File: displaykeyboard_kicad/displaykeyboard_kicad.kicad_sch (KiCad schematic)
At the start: 22 parts, among them SW1 SW_PUSH, SW2 SW_PUSH, SW3 SW_PUSH, SW4 SW_PUSH, SW5 SW_PUSH, SW6 SW_PUSH, SW7 SW_PUSH, SW8 SW_PUSH, SW9 SW_PUSH, U0 supermini_RNF52840, U1 TCA9548APWR, U2 TCA9548APWR, U3 MCP73871

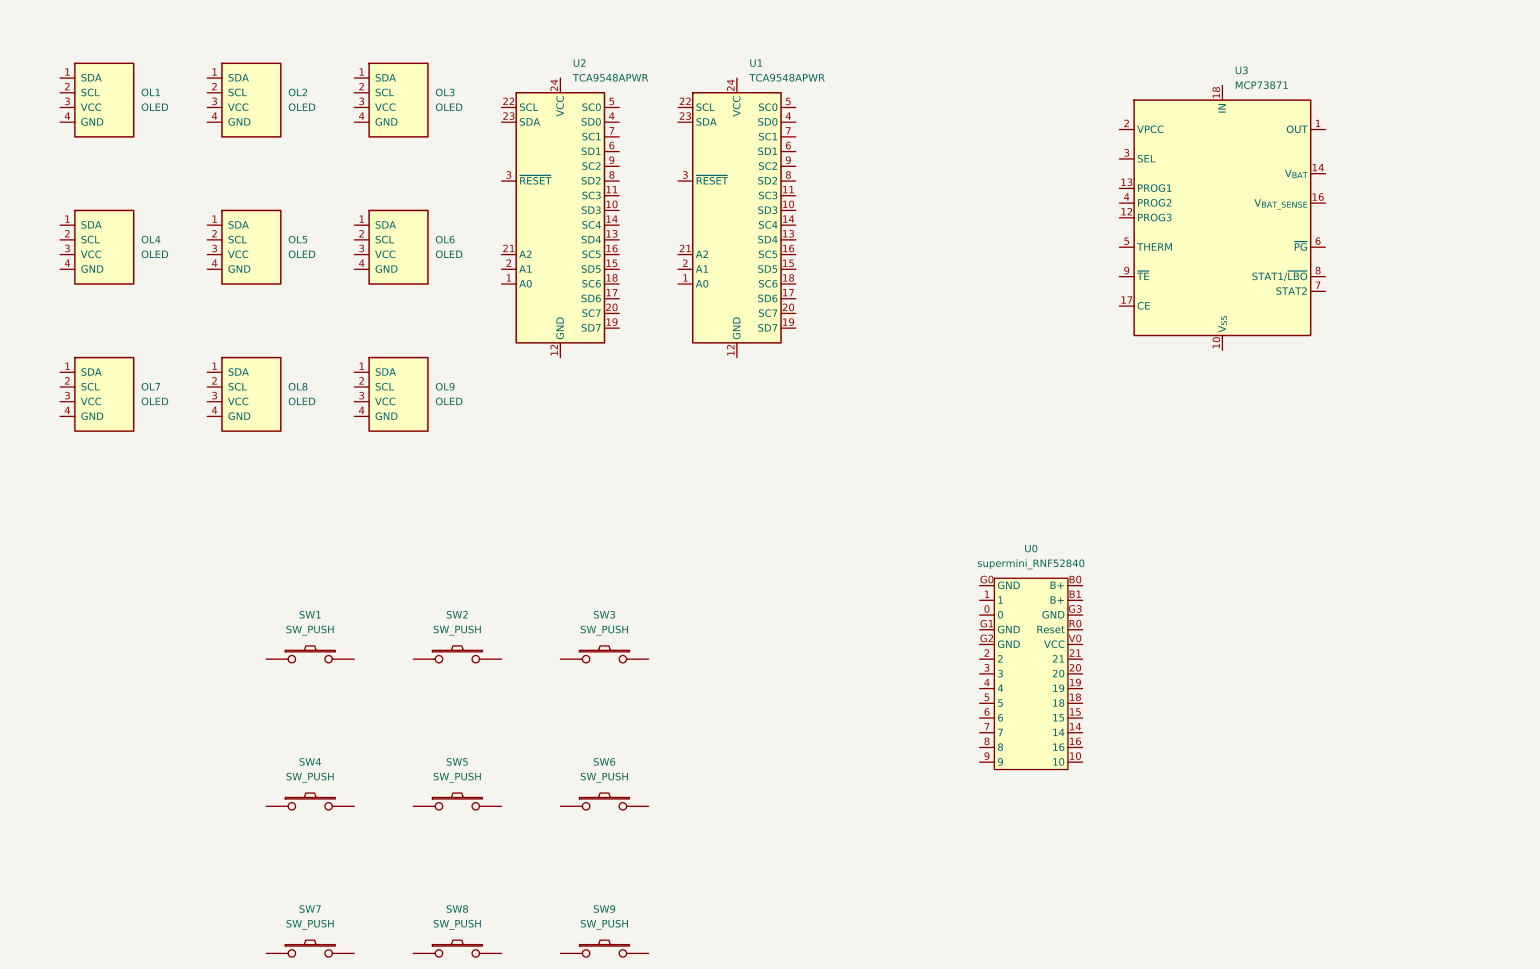
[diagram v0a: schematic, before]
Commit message: main
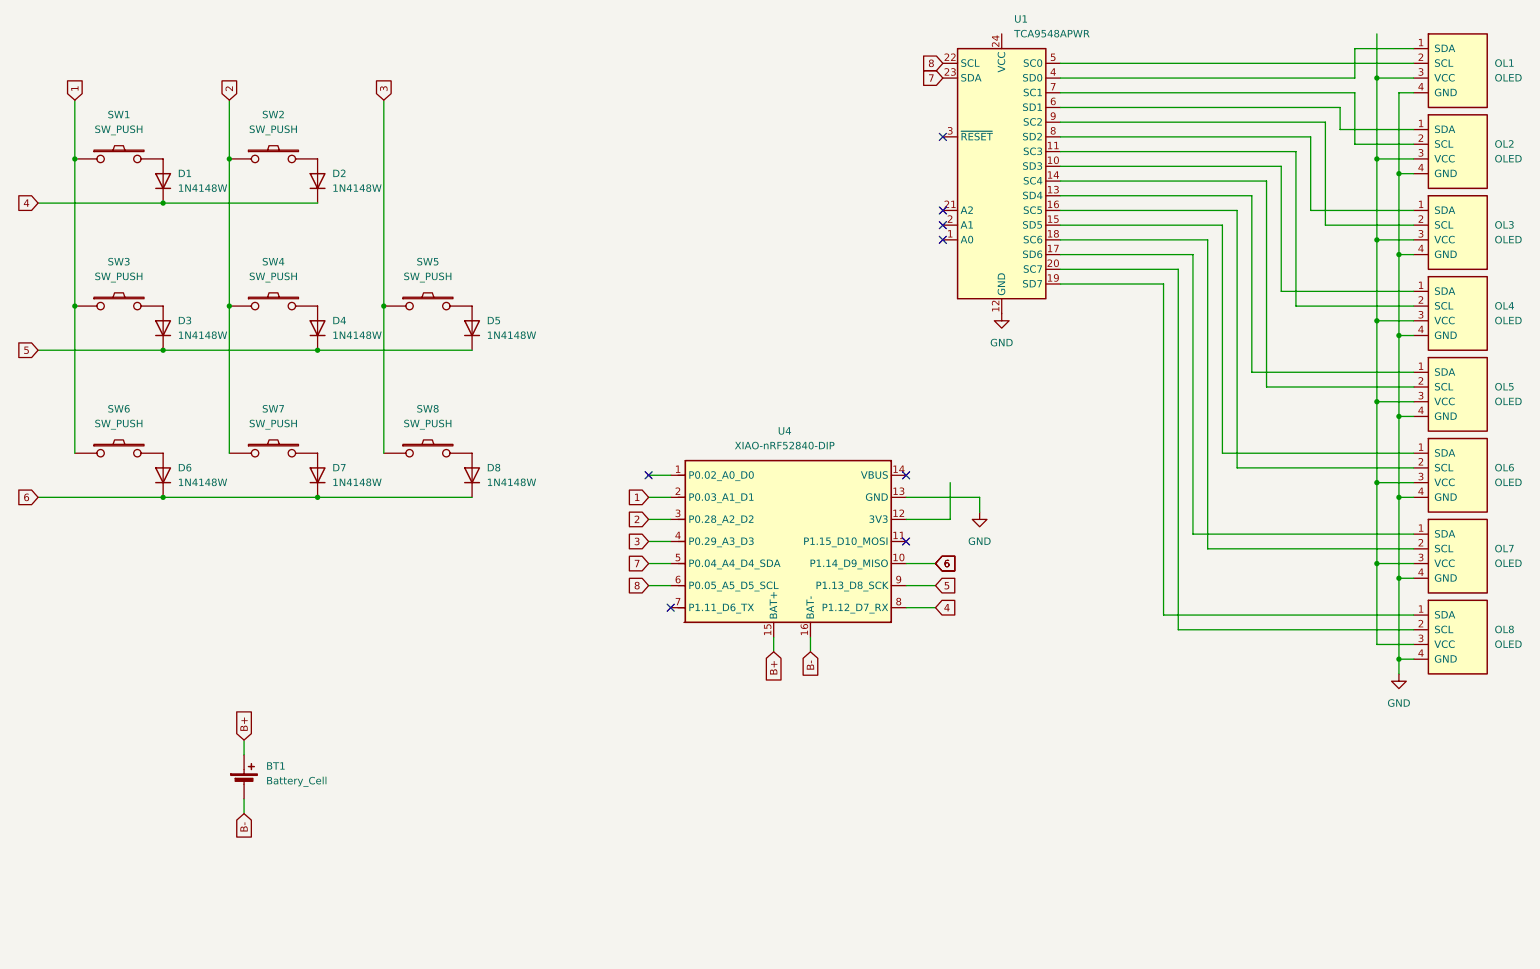
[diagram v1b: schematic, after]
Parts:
- removed OL9: OLED, symbol BrownSugar_KBD:OLED
- removed SW9: SW_PUSH, symbol BrownSugar_KBD:SW_PUSH
- removed U0: supermini_RNF52840, symbol superMini:supermini_NRF52840
- removed U2: TCA9548APWR, Package_SO:TSSOP-24_4.4x7.8mm_P0.65mm, symbol Interface_Expansion:TCA9548APWR
- removed U3: MCP73871, Package_DFN_QFN:QFN-20-1EP_4x4mm_P0.5mm_EP2.5x2.5mm, symbol Battery_Management:MCP73871
- added BT1: Battery_Cell, symbol Device:Battery_Cell
- added D1, D2, D3, D4, D5, D6, D7, D8: 1N4148W, Diode_SMD:D_SOD-123, symbol Diode:1N4148W
- added U4: XIAO-nRF52840-DIP, Seeed_Studio_XIAO_Series:XIAO-nRF52840-DIP, symbol Seeed_Studio_XIAO_Series:XIAO-nRF52840-DIP
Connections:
- net at OL6.1 (SDA): now also U1.15 (SD5)
- net at OL6.2 (SCL): now also U1.16 (SC5)
- net at OL6.3 (VCC): now also OL1.3 (VCC), OL2.3 (VCC), OL3.3 (VCC), OL4.3 (VCC), OL5.3 (VCC), OL7.3 (VCC), OL8.3 (VCC)
- net GND: now reaches OL6.4 (GND)
- net GND: now also OL1.4 (GND), OL2.4 (GND), OL3.4 (GND), OL4.4 (GND), OL5.4 (GND), OL7.4 (GND), OL8.4 (GND), U1.12 (GND), U4.13 (GND)
- net at OL7.1 (SDA): now also U1.17 (SD6)
- net at OL7.2 (SCL): now also U1.18 (SC6)
- net at OL3.1 (SDA): now also U1.8 (SD2)
- net at OL3.2 (SCL): now also U1.9 (SC2)
- net 1: now reaches SW1.1
- net 1: now also SW3.1, SW6.1, U4.2 (P0.03_A1_D1)
- net at SW1.2: now also D1.2 (A)
- net at OL5.1 (SDA): now also U1.13 (SD4)
- net at OL5.2 (SCL): now also U1.14 (SC4)
- net at SW6.2: now also D6.2 (A)
- net at SW3.2: now also D3.2 (A)
- net 3: now reaches SW8.1
- net 3: now also SW5.1, U4.4 (P0.29_A3_D3)
- net at SW8.2: now also D8.2 (A)
- net 2: now reaches SW4.1
- net 2: now also SW2.1, SW7.1, U4.3 (P0.28_A2_D2)
- net at SW4.2: now also D4.2 (A)
- net at OL2.1 (SDA): now also U1.6 (SD1)
- net at OL2.2 (SCL): now also U1.7 (SC1)
- net at SW5.2: now also D5.2 (A)
- net at SW2.2: now also D2.2 (A)
- net at OL1.1 (SDA): now also U1.4 (SD0)
- net at OL1.2 (SCL): now also U1.5 (SC0)
- net at SW7.2: now also D7.2 (A)
- net at U1.10 (SD3): now also OL4.1 (SDA)
- net at U1.11 (SC3): now also OL4.2 (SCL)
- net at U1.19 (SD7): now also OL8.1 (SDA)
- net at U1.20 (SC7): now also OL8.2 (SCL)
- net 8: now reaches U1.22 (SCL)
- net 8: now also U4.6 (P0.05_A5_D5_SCL)
- net 7: now reaches U1.23 (SDA)
- net 7: now also U4.5 (P0.04_A4_D4_SDA)
- new net 4: D1.1 (K), D2.1 (K), U4.8 (P1.12_D7_RX)
- new net 5: D3.1 (K), D4.1 (K), D5.1 (K), U4.9 (P1.13_D8_SCK)
- new net 6: D6.1 (K), D7.1 (K), D8.1 (K), U4.10 (P1.14_D9_MISO)
- new net B+: BT1.1 (+), U4.15 (BAT+)
- new net B-: BT1.2 (-), U4.16 (BAT-)
- no-connect marks 0 -> 8
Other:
- moved on the sheet: OL1, OL2, OL3, OL4, OL5, OL6, SW1, SW2, U1
